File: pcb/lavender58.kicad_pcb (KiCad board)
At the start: 2 copper layers, 195.1 x 126.8 mm, 132 parts, among them U1 xiao-ble, U2 xiao-ble

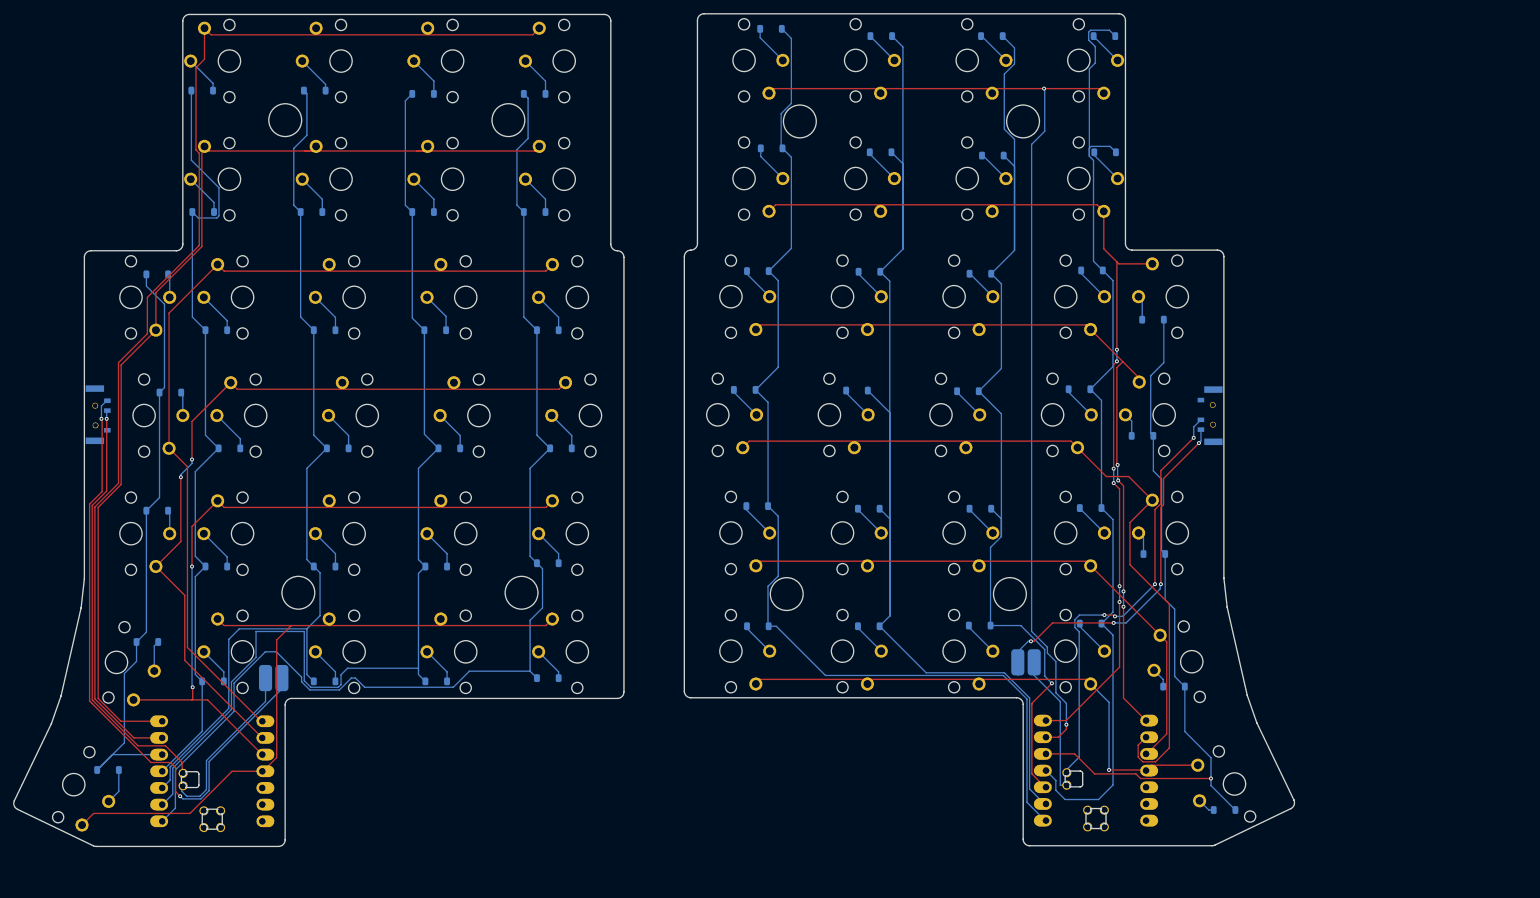
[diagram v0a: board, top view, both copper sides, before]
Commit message: finished lavender58 board
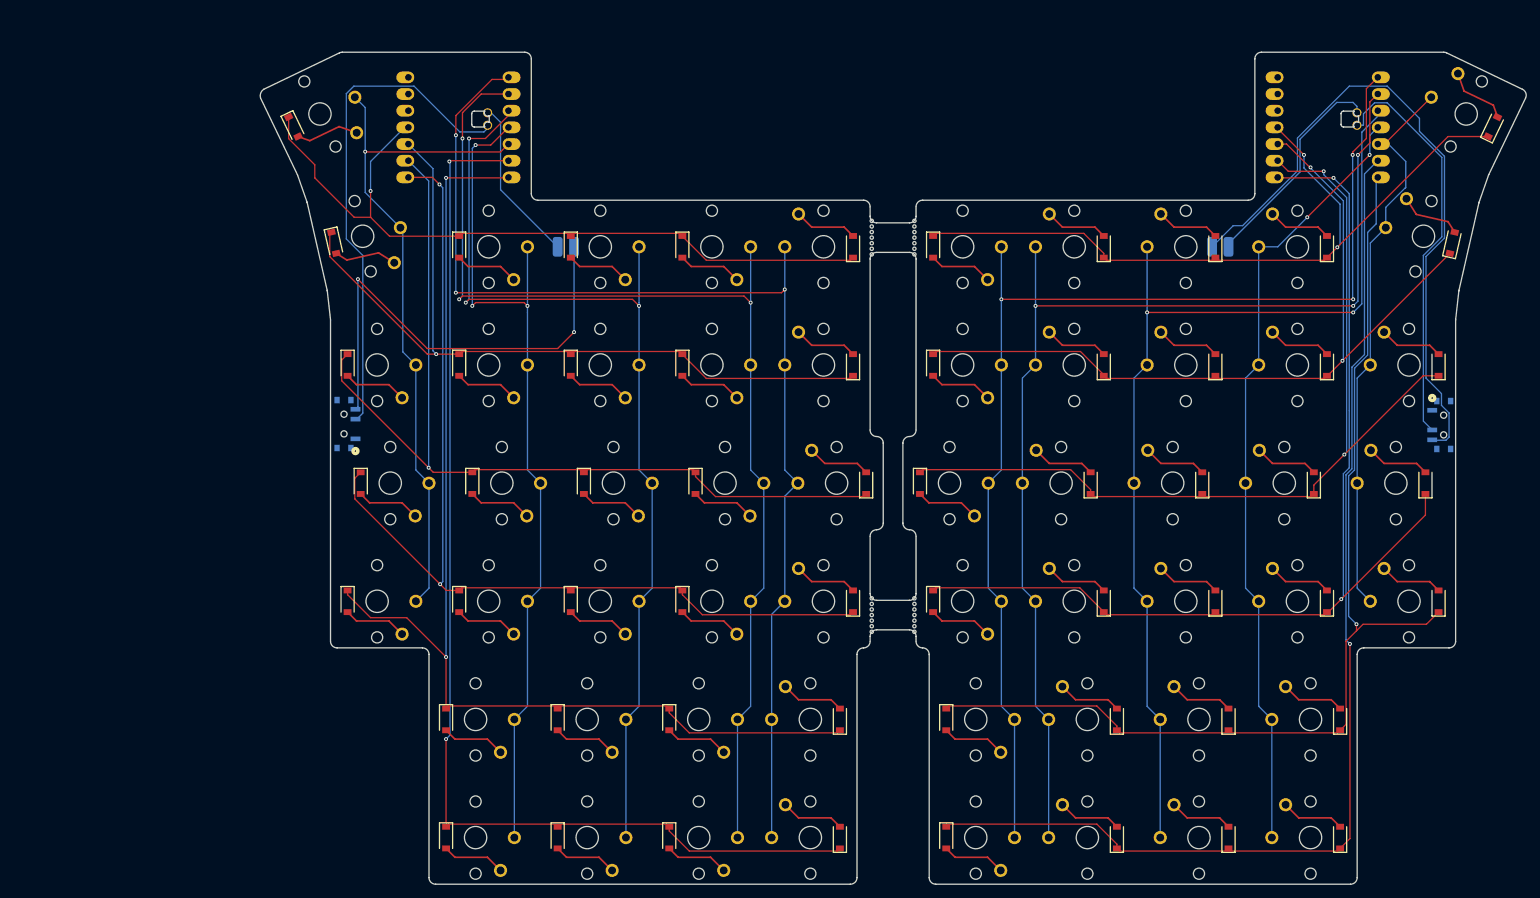
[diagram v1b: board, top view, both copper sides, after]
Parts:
- removed ? (x8): , 
- removed DL1, DL10, DL11, DL12, DL13, DL14, DL15, DL16, DL17, DL18, DL19, DL2, DL20, DL21, DL22, DL23, DL24, DL25, DL26, DL27, DL28, DL29, DL3, DL4, DL5, DL6, DL7, DL8, DL9, DR1, DR10, DR11, DR12, DR13, DR14, DR15, DR16, DR17, DR18, DR19, DR2, DR20, DR21, DR22, DR23, DR24, DR25, DR26, DR27, DR28, DR29, DR3, DR4, DR5, DR6, DR7, DR8, DR9: D_Small, Diode_SMD:D_SOD-123
- removed SWL1, SWL10, SWL11, SWL12, SWL13, SWL14, SWL15, SWL16, SWL17, SWL18, SWL19, SWL2, SWL20, SWL21, SWL22, SWL23, SWL24, SWL25, SWL26, SWL27, SWL28, SWL29, SWL3, SWL4, SWL5, SWL6, SWL7, SWL8, SWL9, SWR1, SWR10, SWR11, SWR12, SWR13, SWR14, SWR15, SWR16, SWR17, SWR18, SWR19, SWR2, SWR20, SWR21, SWR22, SWR23, SWR24, SWR25, SWR26, SWR27, SWR28, SWR29, SWR3, SWR4, SWR5, SWR6, SWR7, SWR8, SWR9: SW_Push_45deg, PCM_marbastlib-choc:SW_choc_v1_1u
- added KL1: diode-choc, lavender58lib:pg1350-D, F.Cu at (175.1, 148.9)
- added KL10: diode-choc, lavender58lib:pg1350-D, F.Cu at (188.1, 94.9)
- added KL11: diode-choc, lavender58lib:pg1350-D, F.Cu at (190.1, 76.9)
- added KL12: diode-choc, lavender58lib:pg1350-D, F.Cu at (190.1, 58.9)
- added KL13: diode-choc, lavender58lib:pg1350-D, F.Cu at (209.1, 148.9)
- added KL14: diode-choc, lavender58lib:pg1350-D, F.Cu at (209.1, 130.9)
- added KL15: diode-choc, lavender58lib:pg1350-D, F.Cu at (207.1, 112.9)
- added KL16: diode-choc, lavender58lib:pg1350-D, F.Cu at (205.1, 94.9)
- added KL17: diode-choc, lavender58lib:pg1350-D, F.Cu at (207.1, 76.9)
- added KL18: diode-choc, lavender58lib:pg1350-D, F.Cu at (207.1, 58.9)
- added KL19: diode-choc, lavender58lib:pg1350-D, F.Cu at (226.1, 148.9)
- added KL2: diode-choc, lavender58lib:pg1350-D, F.Cu at (175.1, 130.9)
- added KL20: diode-choc, lavender58lib:pg1350-D, F.Cu at (226.1, 130.9)
- added KL21: diode-choc, lavender58lib:pg1350-D, F.Cu at (224.1, 112.9)
- added KL22: diode-choc, lavender58lib:pg1350-D, F.Cu at (222.1, 94.9)
- added KL23: diode-choc, lavender58lib:pg1350-D, F.Cu at (224.1, 76.9)
- added KL24: diode-choc, lavender58lib:pg1350-D, F.Cu at (224.1, 58.9)
- added KL25: diode-choc, lavender58lib:pg1350-D, F.Cu at (241.1, 112.9)
- added KL26: diode-choc, lavender58lib:pg1350-D, F.Cu at (239.1, 94.9)
- added KL27: diode-choc, lavender58lib:pg1350-D, F.Cu at (241.1, 76.9)
- added KL28: diode-choc, lavender58lib:pg1350-D, F.Cu at (243.3, 57.3)
- added KL29: diode-choc, lavender58lib:pg1350-D, F.Cu at (249.8, 38.7)
- added KL3: diode-choc, lavender58lib:pg1350-D, F.Cu at (173.1, 112.9)
- added KL4: diode-choc, lavender58lib:pg1350-D, F.Cu at (171.1, 94.9)
- added KL5: diode-choc, lavender58lib:pg1350-D, F.Cu at (173.1, 76.9)
- added KL6: diode-choc, lavender58lib:pg1350-D, F.Cu at (173.1, 58.9)
- added KL7: diode-choc, lavender58lib:pg1350-D, F.Cu at (192.1, 148.9)
- added KL8: diode-choc, lavender58lib:pg1350-D, F.Cu at (192.1, 130.9)
- added KL9: diode-choc, lavender58lib:pg1350-D, F.Cu at (190.1, 112.9)
- added KR1: diode-choc, lavender58lib:pg1350-D, F.Cu at (149.9, 148.9)
- added KR10: diode-choc, lavender58lib:pg1350-D, F.Cu at (136.9, 94.9)
- added KR11: diode-choc, lavender58lib:pg1350-D, F.Cu at (134.9, 76.9)
- added KR12: diode-choc, lavender58lib:pg1350-D, F.Cu at (134.9, 58.9)
- added KR13: diode-choc, lavender58lib:pg1350-D, F.Cu at (115.9, 148.9)
- added KR14: diode-choc, lavender58lib:pg1350-D, F.Cu at (115.9, 130.9)
- added KR15: diode-choc, lavender58lib:pg1350-D, F.Cu at (117.9, 112.9)
- added KR16: diode-choc, lavender58lib:pg1350-D, F.Cu at (119.9, 94.9)
- added KR17: diode-choc, lavender58lib:pg1350-D, F.Cu at (117.9, 76.9)
- added KR18: diode-choc, lavender58lib:pg1350-D, F.Cu at (117.9, 58.9)
- added KR19: diode-choc, lavender58lib:pg1350-D, F.Cu at (98.9, 148.9)
- added KR2: diode-choc, lavender58lib:pg1350-D, F.Cu at (149.9, 130.9)
- added KR20: diode-choc, lavender58lib:pg1350-D, F.Cu at (98.9, 130.9)
- added KR21: diode-choc, lavender58lib:pg1350-D, F.Cu at (100.9, 112.9)
- added KR22: diode-choc, lavender58lib:pg1350-D, F.Cu at (102.9, 94.9)
- added KR23: diode-choc, lavender58lib:pg1350-D, F.Cu at (100.9, 76.9)
- added KR24: diode-choc, lavender58lib:pg1350-D, F.Cu at (100.9, 58.9)
- added KR25: diode-choc, lavender58lib:pg1350-D, F.Cu at (83.9, 112.9)
- added KR26: diode-choc, lavender58lib:pg1350-D, F.Cu at (85.9, 94.9)
- added KR27: diode-choc, lavender58lib:pg1350-D, F.Cu at (83.9, 76.9)
- added KR28: diode-choc, lavender58lib:pg1350-D, F.Cu at (81.7, 57.3)
- added KR29: diode-choc, lavender58lib:pg1350-D, F.Cu at (75.2, 38.7)
- added KR3: diode-choc, lavender58lib:pg1350-D, F.Cu at (151.9, 112.9)
- added KR4: diode-choc, lavender58lib:pg1350-D, F.Cu at (153.9, 94.9)
- added KR5: diode-choc, lavender58lib:pg1350-D, F.Cu at (151.9, 76.9)
- added KR6: diode-choc, lavender58lib:pg1350-D, F.Cu at (151.9, 58.9)
- added KR7: diode-choc, lavender58lib:pg1350-D, F.Cu at (132.9, 148.9)
- added KR8: diode-choc, lavender58lib:pg1350-D, F.Cu at (132.9, 130.9)
- added KR9: diode-choc, lavender58lib:pg1350-D, F.Cu at (134.9, 112.9)
- added REF**: MouseBite-Part_2.0x4.5mm_outset_D0.5mm_P0.85mm_7h, Panelization:MouseBite-Part_2.0x4.5mm_outset_D0.5mm_P0.85mm_7h, F.Cu at (166.0, 57.5)
- added REF**: MouseBite-Part_2.0x4.5mm_outset_D0.5mm_P0.85mm_7h, Panelization:MouseBite-Part_2.0x4.5mm_outset_D0.5mm_P0.85mm_7h, F.Cu at (159.0, 57.5)
- added REF**: MouseBite-Part_2.0x4.5mm_outset_D0.5mm_P0.85mm_7h, Panelization:MouseBite-Part_2.0x4.5mm_outset_D0.5mm_P0.85mm_7h, F.Cu at (159.0, 115.0)
- added REF**: MouseBite-Part_2.0x4.5mm_outset_D0.5mm_P0.85mm_7h, Panelization:MouseBite-Part_2.0x4.5mm_outset_D0.5mm_P0.85mm_7h, F.Cu at (166.0, 115.0)
- +: renamed from BAT+1; footprint Connector_Wire:SolderWirePad_1x01_SMD_2x4mm -> Connector_Wire:SolderWirePad_1x01_SMD_1.5x3mm
- +: renamed from BAT+2; footprint Connector_Wire:SolderWirePad_1x01_SMD_2x4mm -> Connector_Wire:SolderWirePad_1x01_SMD_1.5x3mm
- -: renamed from BATGND1; footprint Connector_Wire:SolderWirePad_1x01_SMD_2x4mm -> Connector_Wire:SolderWirePad_1x01_SMD_1.5x3mm
- -: renamed from BATGND2; footprint Connector_Wire:SolderWirePad_1x01_SMD_2x4mm -> Connector_Wire:SolderWirePad_1x01_SMD_1.5x3mm
- PSW1, PSW2: footprint TOTEMlib:MSK12C02 -> lavender58lib:CUS-12TB_NDC
- U1, U2: footprint TOTEMlib:xiao-ble-smd-cutout -> lavender58lib:xiao-ble-smd-cutout-2
- moved PSW1 206.8 mm to (246.4, 86.0), turned to -90 degrees
- moved U1 196.2 mm to (228.7, 40.7), turned to 180 degrees
- moved - 160.7 mm to (213.6, 58.9)
- moved + 156.2 mm to (211.1, 58.9), turned to 0 degrees
- moved U2 138.0 mm to (96.3, 40.7), turned to 180 degrees
- moved PSW2 133.8 mm to (78.9, 85.9), turned to 90 degrees
- moved - 96.3 mm to (111.4, 58.9), turned to 180 degrees
- moved + 92.6 mm to (113.9, 58.9), turned to 180 degrees
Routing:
- net COL4_R: track 86.4 -> 125.5 mm, vias 0 -> 1
- net COL5_R: track 79.7 -> 115.1 mm
- net COL2_R: track 120.1 -> 155.0 mm, vias 4 -> 2
- net ROW1_R: track 206.1 -> 174.3 mm, vias 0 -> 3
- net COL2_L: track 130.5 -> 160.8 mm, vias 0 -> 2
- net COL1_R: track 142.8 -> 172.4 mm, vias 6 -> 2
- net COL3_L: track 117.4 -> 142.1 mm
- net COL3_R: track 117.6 -> 140.6 mm, vias 0 -> 1
- net ROW2_L: track 135.9 -> 156.2 mm, vias 0 -> 2
- net COL4_L: track 106.9 -> 126.6 mm
- net ROW0_R: track 162.2 -> 180.5 mm, vias 0 -> 3
- net COL0_R: track 155.9 -> 173.1 mm
- net VBAT_R: track 56.1 -> 71.3 mm, vias 4 -> 2
- net ROW3_R: track 145.4 -> 132.1 mm, vias 0 -> 3
- net ROW1_L: track 161.6 -> 174.7 mm, vias 0 -> 3
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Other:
- board size 195.1 x 126.8 mm -> 192.9 x 126.7 mm
